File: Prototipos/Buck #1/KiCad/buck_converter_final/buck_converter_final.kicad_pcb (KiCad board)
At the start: 2 copper layers, 100 x 100 mm, 25 parts, among them J1 Conn_01x03_Pin, J2 Screw_Terminal_01x02, J3 Screw_Terminal_01x02, Q1 IRF9540NPBF, Q3 NPN

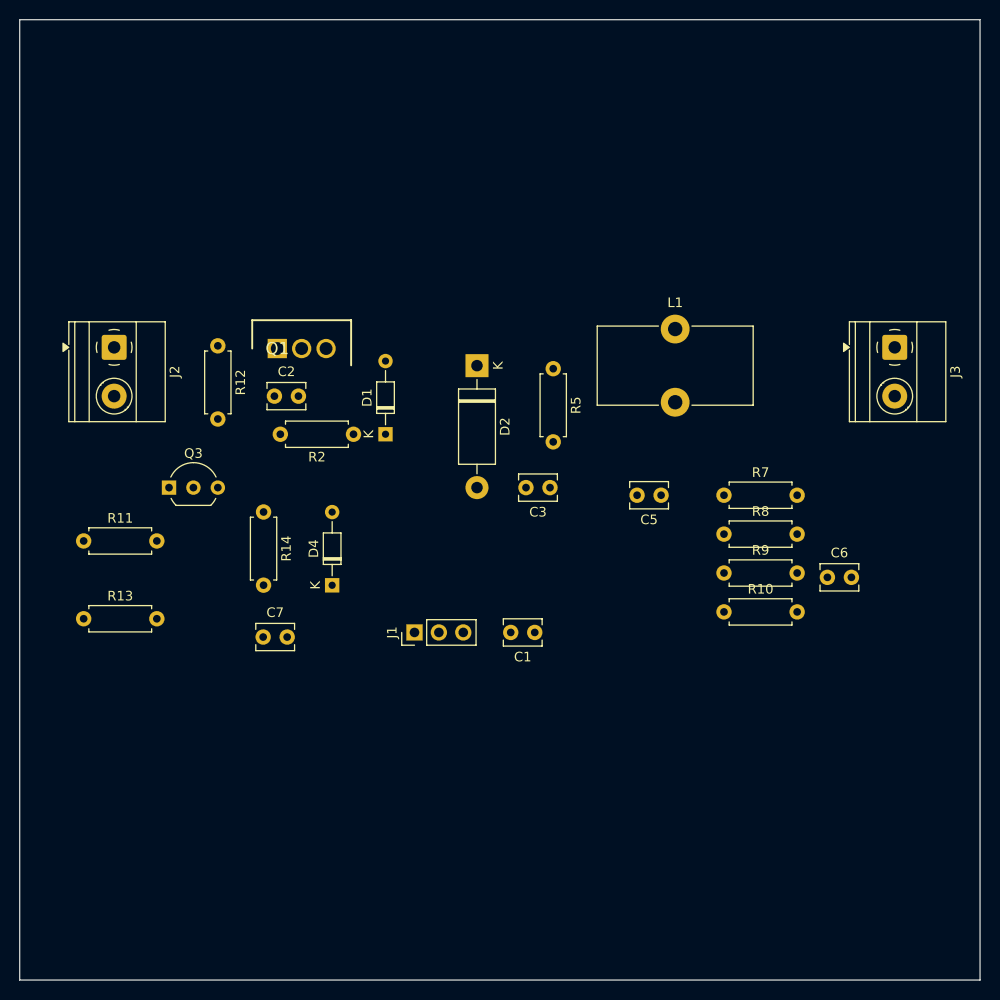
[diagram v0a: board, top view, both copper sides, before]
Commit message: Primera versión PCB final Buck
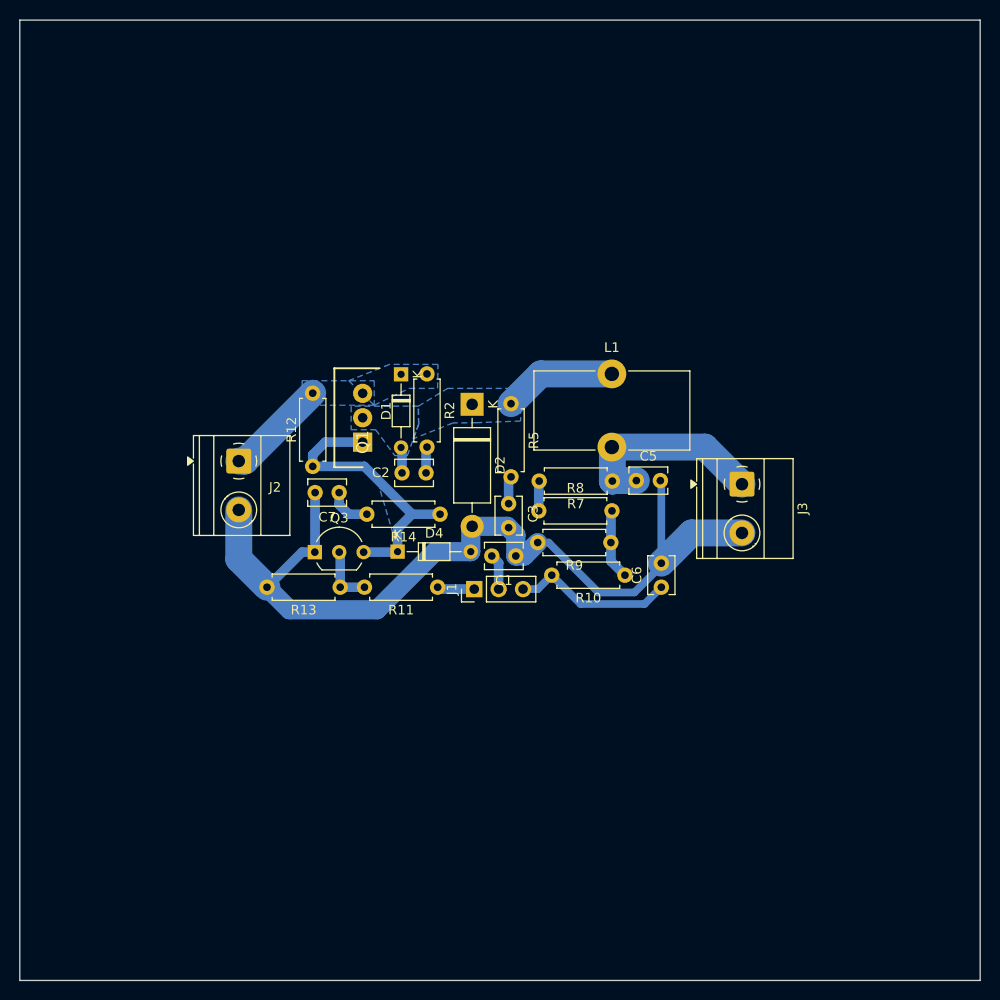
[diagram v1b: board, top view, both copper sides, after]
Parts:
- moved R11 37.2 mm to (148.3, 91.7), turned to 180 degrees
- moved R13 26.9 mm to (138.2, 91.7), turned to 180 degrees
- moved J3 21.4 mm to (180.0, 80.9)
- moved R8 19.4 mm to (158.8, 83.7)
- moved R14 18.4 mm to (148.6, 84.0), turned to 180 degrees
- moved C2 17.7 mm to (147.1, 79.8), turned to 180 degrees
- moved J2 17.6 mm to (127.6, 78.5)
- moved C6 17.3 mm to (171.6, 91.7), turned to 90 degrees
- moved C7 17.0 mm to (138.1, 81.8), turned to 180 degrees
- moved Q3 16.6 mm to (135.5, 88.0)
- moved Q1 13.2 mm to (140.5, 76.5), turned to 90 degrees
- moved R9 12.2 mm to (166.3, 87.0), turned to 180 degrees
- moved R7 11.7 mm to (166.5, 80.6), turned to 180 degrees
- moved R12 11.0 mm to (135.3, 71.5)
- moved R10 11.0 mm to (167.8, 90.4), turned to 180 degrees
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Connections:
- J1 pad 2: RETRO_MICRO -> AGND
- J1 pad 3: AGND -> RETRO_MICRO
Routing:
- net PGND: track 0.00 -> 94.1 mm
- net Gate: track 0.00 -> 30.4 mm
- net Net-(J3-Pin_1): track 0.00 -> 21.2 mm
- net RETRO_MICRO: track 0.00 -> 17.0 mm
- net Net-(D1-A): track 0.00 -> 14.5 mm
- net 12V: track 0.00 -> 10.6 mm
- net Net-(R10-Pad1): track 0.00 -> 7.35 mm
- net Net-(Q3-B): track 0.00 -> 6.22 mm
- net Net-(C7-Pad1): track 0.00 -> 4.82 mm
- net PWM_CONTROL: track 0.00 -> 3.89 mm
- net AGND: track 0.00 -> 3.74 mm
- net Net-(R7-Pad2): track 0.00 -> 3.12 mm
- net Net-(C3-Pad1): track 0.00 -> 2.89 mm
- net Net-(C2-Pad1): track 0.00 -> 2.73 mm
- added copper zone on B.Cu, net 12V
- added copper zone on B.Cu, net Gate
- added copper zone on B.Cu, net Net-(D1-A)
